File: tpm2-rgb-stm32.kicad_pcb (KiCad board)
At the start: 4 copper layers, 1 x 0.7 mm, 59 parts, among them J1 Screw_Terminal_01x04, J2 Screw_Terminal_01x04, J3 Screw_Terminal_01x02, J4 Screw_Terminal_01x02, J5 12401832E402A, J6 Screw_Terminal_01x04, SW1 SW_Push, U1 COS4426SR, U10 IRF7458TRPBF, U11 IRF7458TRPBF, U12 COS4426SR, U13 IRF7458TRPBF, U14 IRF7458TRPBF, U15 FT232RL, U2 IRF7458TRPBF, U3 IRF7458TRPBF, U4 STM32F103CBTx, U5 COS4426SR, U6 IRF7458TRPBF, U7 IRF7458TRPBF, U8 COS4426SR, U9 LM1117-3.3, Y1 8MHz

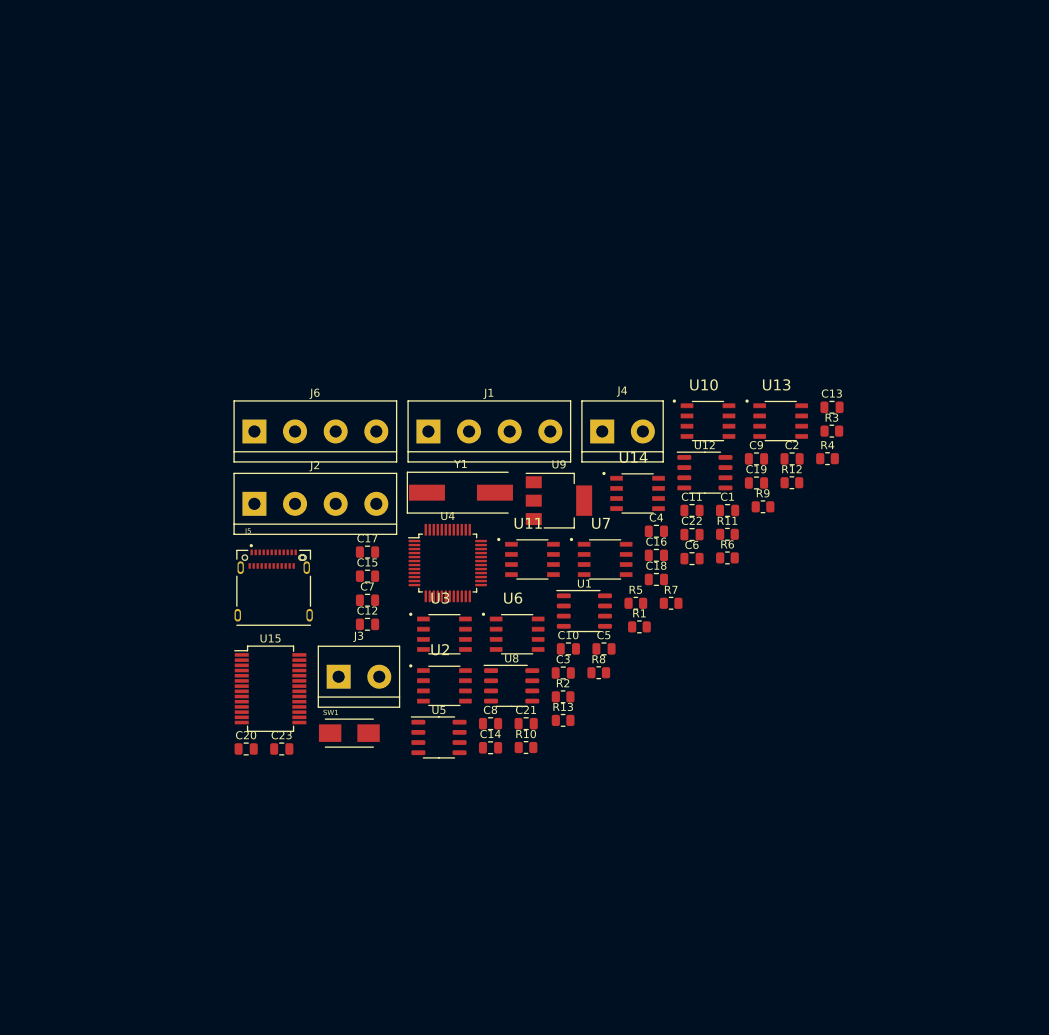
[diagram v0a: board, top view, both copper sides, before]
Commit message: Start layout
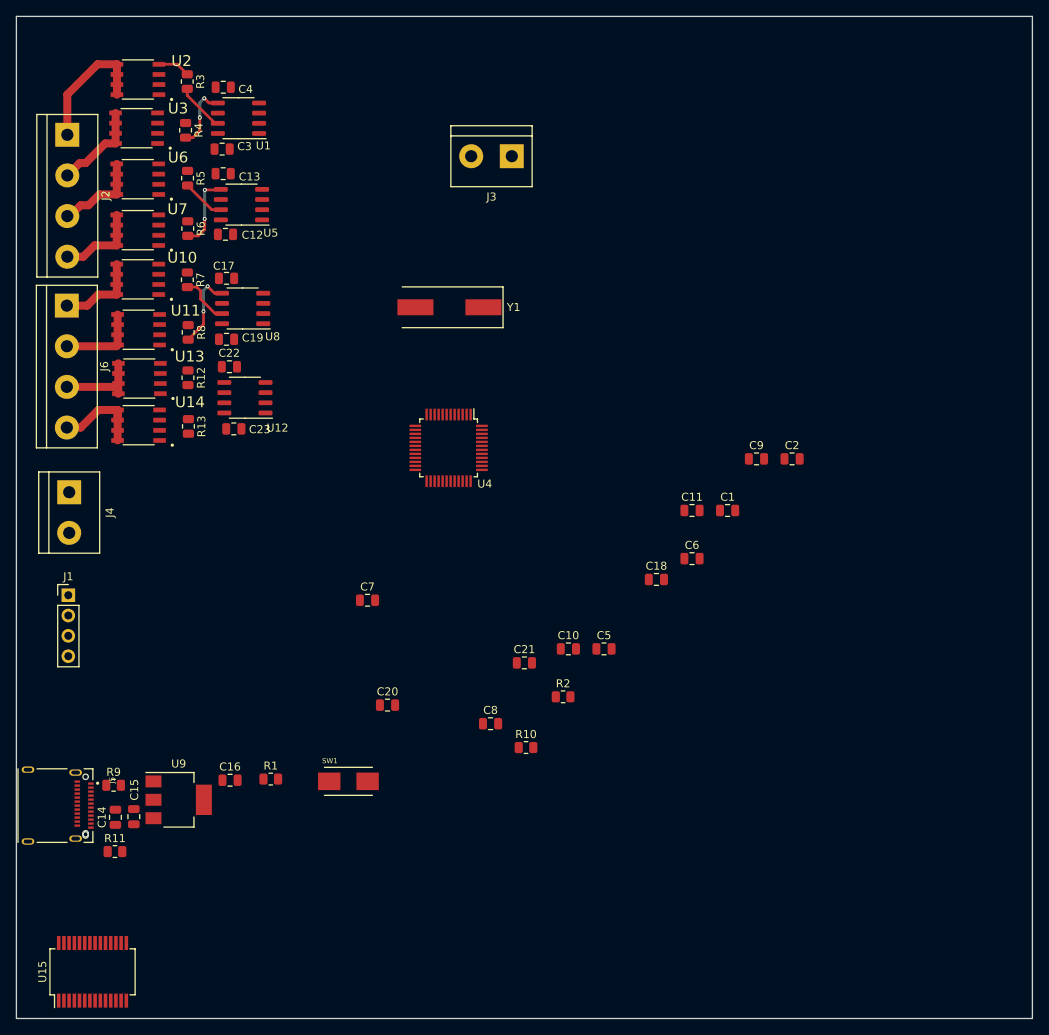
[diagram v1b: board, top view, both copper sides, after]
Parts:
- J1: value Screw_Terminal_01x04 -> Conn_01x04_Male; footprint TerminalBlock:TerminalBlock_bornier-4_P5.08mm -> Connector_PinHeader_2.54mm:PinHeader_1x04_P2.54mm_Vertical
- moved R3 91.7 mm to (34.1, 9.88), turned to -90 degrees
- moved R4 90.1 mm to (33.8, 16.0), turned to -90 degrees
- moved R9 88.3 mm to (24.9, 97.8)
- moved R11 86.2 mm to (25.0, 106.1)
- moved U2 84.9 mm to (27.9, 9.63), turned to 180 degrees
- moved C13 81.5 mm to (38.5, 21.4)
- moved U13 80.4 mm to (28.1, 47.0), turned to 180 degrees
- moved R6 79.0 mm to (34.1, 28.3), turned to -90 degrees
- moved C3 78.1 mm to (38.4, 18.3)
- moved C4 77.5 mm to (38.6, 10.6)
- moved R5 77.2 mm to (34.1, 22.0), turned to -90 degrees
- moved R12 76.6 mm to (34.1, 46.9), turned to -90 degrees
- moved U1 75.3 mm to (40.5, 14.5), turned to 180 degrees
- moved U6 74.1 mm to (27.9, 22.1), turned to 180 degrees
- moved U3 74.0 mm to (27.7, 15.7), turned to 180 degrees
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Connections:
- J1 pad 1: +5V -> GND
- J1 pad 2: SWDIO -> SWDCLK
- J1 pad 3: SWDCLK -> SWDIO
- J1 pad 4: GND -> +5V
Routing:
- net OUT1: track 0.00 -> 16.6 mm
- net OUT8: track 0.00 -> 12.3 mm
- net OUT2: track 0.00 -> 11.5 mm
- net OUT3: track 0.00 -> 11.1 mm
- net OUT5: track 0.00 -> 10.6 mm
- net OUT4: track 0.00 -> 10.6 mm
- net OUT7: track 0.00 -> 10.4 mm
- net OUT6: track 0.00 -> 10.2 mm
- net GATE6: track 0.00 -> 9.84 mm, vias 0 -> 2
- net GATE4: track 0.00 -> 9.43 mm, vias 0 -> 2
- net GATE2: track 0.00 -> 8.37 mm, vias 0 -> 2
- net GATE5: track 0.00 -> 6.31 mm
- net GATE1: track 0.00 -> 6.10 mm
- net GATE3: track 0.00 -> 5.42 mm
- net Net-(R3-Pad1): track 0.00 -> 4.06 mm
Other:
- board size 1 x 0.7 mm -> 127 x 125.3 mm
